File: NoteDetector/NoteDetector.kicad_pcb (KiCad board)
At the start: 2 copper layers, 25 x 25 mm, 24 parts, among them J1 Conn_02x03, J3 Conn_01x01, J4 Conn_01x01, Q1 Q_NMOS_DGS, U1 VM1010, U2 OPAMP, U3 ATtiny1614-SS

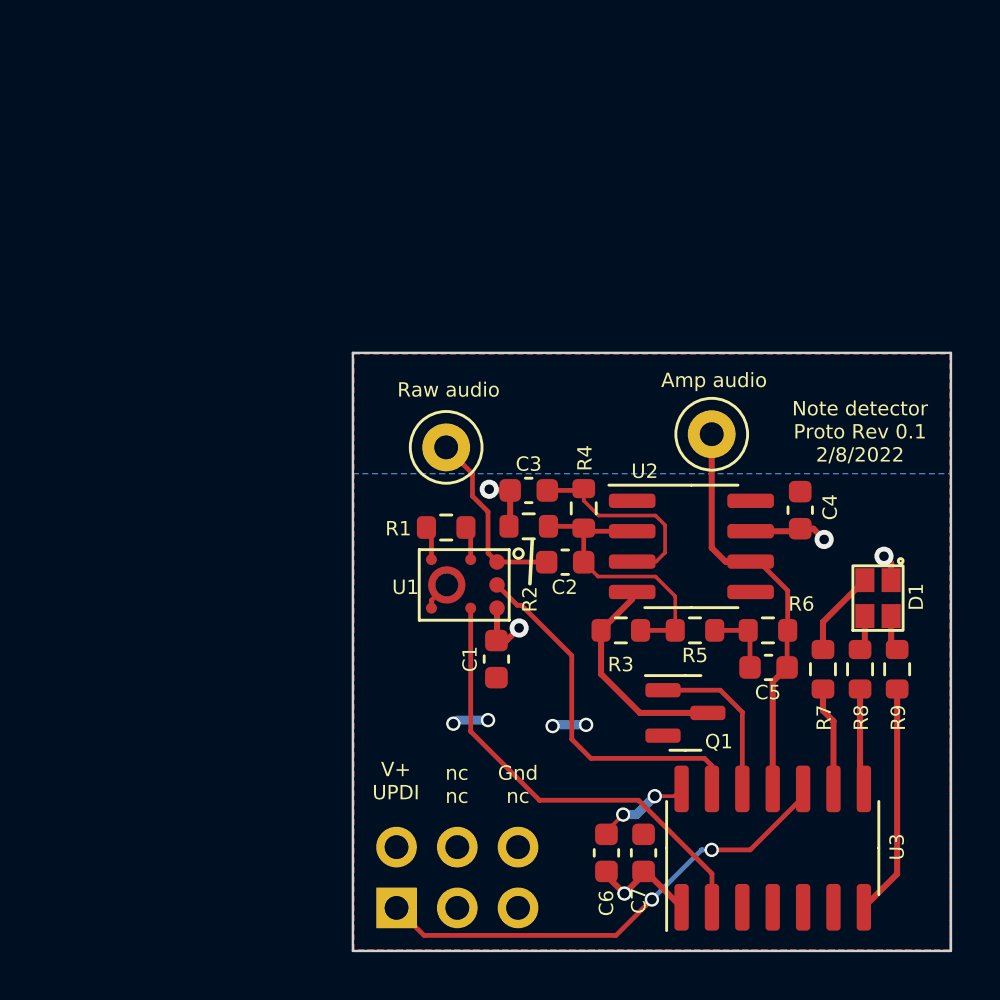
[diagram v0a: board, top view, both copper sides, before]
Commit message: save work: new layout almost done
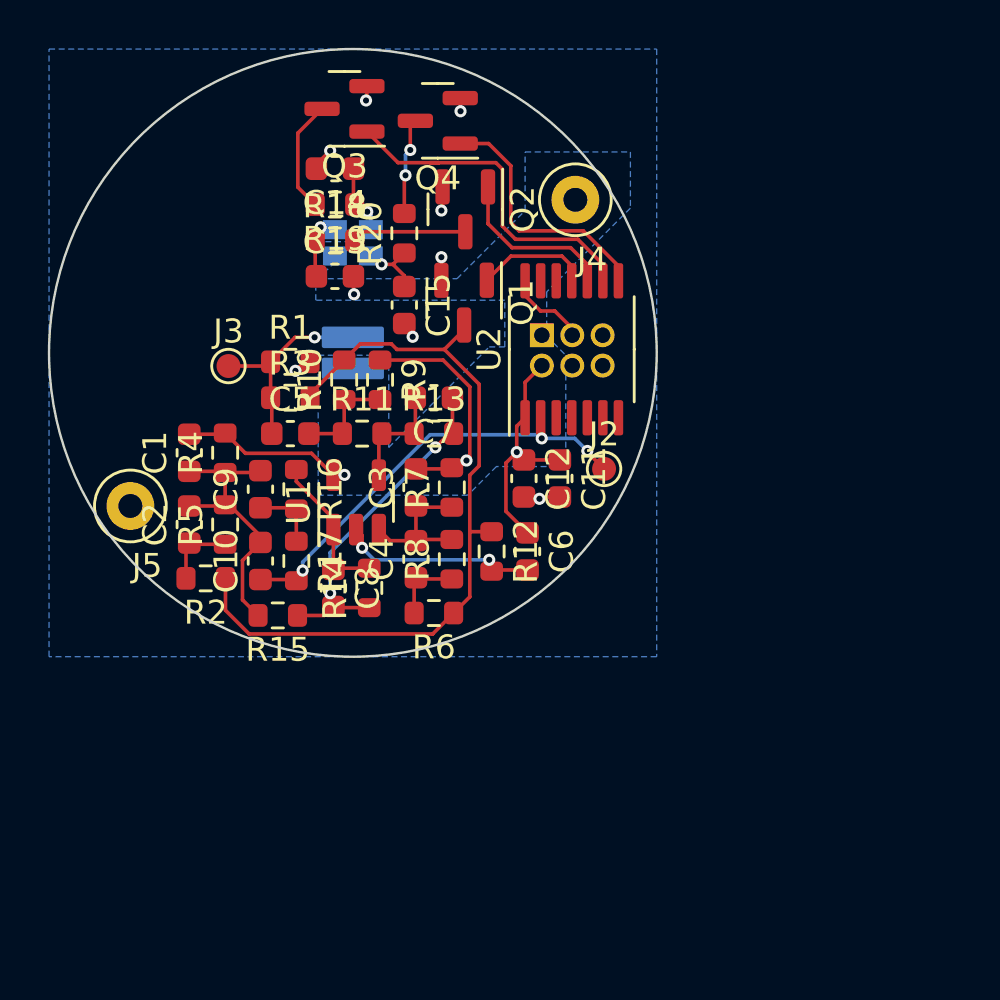
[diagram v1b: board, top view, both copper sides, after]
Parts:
- removed U3: ATtiny1614-SS, Package_SO:SOIC-14_3.9x8.7mm_P1.27mm
- added C10: 22p, Capacitor_SMD:C_0603_1608Metric, F.Cu at (-3.86, 8.70)
- added C11: 100n, Capacitor_SMD:C_0603_1608Metric, F.Cu at (8.65, 5.25)
- added C12: 10n, Capacitor_SMD:C_0603_1608Metric, F.Cu at (7.15, 5.25)
- added C13: 1u, Capacitor_SMD:C_0603_1608Metric, F.Cu at (-0.75, -3.20)
- added C14: 1u, Capacitor_SMD:C_0603_1608Metric, F.Cu at (-0.75, -7.70)
- added C15: 1u, Capacitor_SMD:C_0603_1608Metric, F.Cu at (2.15, -2.00)
- added C8: 22p, Capacitor_SMD:C_0603_1608Metric, F.Cu at (-0.81, 9.82)
- added C9: 22p, Capacitor_SMD:C_0603_1608Metric, F.Cu at (-3.86, 5.70)
- added J2: Conn_01x01, TestPoint:TestPoint_Pad_D1.0mm, F.Cu at (10.5, 4.85)
- added J5: Conn_01x01, TestPoint:TestPoint_Loop_D2.50mm_Drill1.0mm, F.Cu at (-9.30, 6.40)
- added MK1: Microphone_Condenser, User:ElectretCondenserMic_SMT_MO063602-1, B.Cu at (0.00, 0.00)
- added Q2: Q_NMOS_DGS, Package_TO_SOT_SMD:SOT-23, F.Cu at (4.70, -6.00)
- added Q3: Q_NMOS_DGS, Package_TO_SOT_SMD:SOT-23, F.Cu at (-0.35, -10.2)
- added Q4: Q_NMOS_DGS, Package_TO_SOT_SMD:SOT-23, F.Cu at (3.55, -9.70)
- added R10: 10M, Resistor_SMD:R_0603_1608Metric, F.Cu at (-0.36, 1.12)
- added R11: 270k, Resistor_SMD:R_0603_1608Metric, F.Cu at (0.39, 3.38)
- added R12: 100, Resistor_SMD:R_0603_1608Metric, F.Cu at (5.80, 8.30)
- added R13: 10M, Resistor_SMD:R_0603_1608Metric, F.Cu at (3.39, 3.38)
- added R14: 10M, Resistor_SMD:R_0603_1608Metric, F.Cu at (0.69, 9.82)
- added R15: 270k, Resistor_SMD:R_0603_1608Metric, F.Cu at (-3.14, 11.0)
- added R16: 270k, Resistor_SMD:R_0603_1608Metric, F.Cu at (-2.36, 5.70)
- added R17: 270k, Resistor_SMD:R_0603_1608Metric, F.Cu at (-2.36, 8.70)
- added R18: R, Resistor_SMD:R_0603_1608Metric, F.Cu at (-0.75, -4.70)
- added R19: R, Resistor_SMD:R_0603_1608Metric, F.Cu at (-0.75, -6.20)
- added R20: R, Resistor_SMD:R_0603_1608Metric, F.Cu at (2.15, -5.00)
- C1, C4: value 100n -> 1n
- C2: value 1.5n -> 1n
- C3: value C -> 1n
- C5: value 47p -> 100n
- C6: value 100n -> 10n
- C7: value 10n -> 22p
- D1: moved to B.Cu
- J1: value Conn_02x03 -> Conn_01x05; footprint Connector_PinSocket_2.54mm:PinSocket_2x03_P2.54mm_Vertical -> Connector_PinHeader_1.27mm:PinHeader_2x03_P1.27mm_Vertical
- J3: footprint TestPoint:TestPoint_Loop_D2.50mm_Drill1.0mm -> TestPoint:TestPoint_Pad_D1.0mm
- R1: value 18k -> 1k
- R2, R3: value 10M -> 1k
- R5: value 10k -> 10M
- R6: value 1M -> 1k
- R7, R8, R9: value R -> 10M
- U1: value VM1010 -> OPAMP; footprint User:MEMS_mic_VS1010 -> Package_TO_SOT_SMD:SOT-23-5
- U2: value OPAMP -> PIC18F06; footprint Package_SO:SOIC-8_3.9x4.9mm_P1.27mm -> Package_SO:TSSOP-14_4.4x5mm_P0.65mm
- moved D1 26.5 mm to (0.00, -4.60), turned to 180 degrees
- moved R9 24.8 mm to (1.14, 1.12)
- moved J1 24.7 mm to (7.90, -0.74)
- moved C5 22.3 mm to (-2.61, 3.38), turned to 0 degrees
- moved C7 20.9 mm to (3.39, 1.88), turned to 180 degrees
- moved J3 20.4 mm to (-5.20, 0.55)
- moved R5 20.1 mm to (-5.34, 7.17), turned to 90 degrees
- moved Q1 19.5 mm to (4.65, -2.10), turned to -90 degrees
- moved R8 17.7 mm to (4.14, 8.62), turned to 90 degrees
- moved R7 17.3 mm to (4.14, 5.62), turned to 90 degrees
- moved R3 16.9 mm to (-2.61, 1.88), turned to 0 degrees
- moved C4 16.2 mm to (2.64, 8.62), turned to 90 degrees
- moved C2 15.8 mm to (-6.84, 7.17), turned to 90 degrees
- moved C1 15.5 mm to (-6.84, 4.17)
- moved R4 15.2 mm to (-5.34, 4.17)
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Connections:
- C1 pad 1: GND -> /Midscale2
- C2 pad 1: /Audio_raw -> Net-(C2-Pad1)
- C2 pad 2: Net-(C2-Pad2) -> /Midscale2
- C3 pad 1: Net-(C3-Pad1) -> /Midscale1
- C4 pad 1: GND -> Net-(C4-Pad1)
- C4 pad 2: +BATT -> /Midscale1
- C5 pad 1: /Audio_In -> /Audio_raw
- C6 pad 2: GND -> Net-(C6-Pad2)
- C7 pad 1: +BATT -> Net-(C7-Pad1)
- C7 pad 2: GND -> Net-(C7-Pad2)
- J1 pad 1: /UPDI -> /~{MCLR}
- J1 pad 3: unconnected-(J1-Pad3) -> GND
- J1 pad 4: unconnected-(J1-Pad4) -> /ICSP_DAT
- J1 pad 5: unconnected-(J1-Pad5) -> /ICSP_CLK
- J1 pad 6: GND -> unconnected-(J1-Pad6)
- J3 pad 1: /Audio_In -> /Audio_raw
- J4 pad 1: /Audio_raw -> +BATT
- Q1 pad 3: /AFE_gnd -> /gnd_switch
- R1 pad 1: Net-(R1-Pad1) -> /Audio_raw
- R1 pad 2: Net-(R1-Pad2) -> GND
- R2 pad 1: +BATT -> /gnd_switch
- R2 pad 2: Net-(C2-Pad2) -> Net-(C2-Pad1)
- R3 pad 1: Net-(C2-Pad2) -> /Audio_raw
- R3 pad 2: /AFE_gnd -> /gnd_switch
- R4 pad 1: Net-(C2-Pad2) -> /Midscale2
- R4 pad 2: Net-(C3-Pad1) -> +BATT
- R5 pad 1: Net-(C2-Pad2) -> Net-(C2-Pad1)
- R5 pad 2: Net-(C5-Pad2) -> /Midscale2
- R6 pad 1: Net-(C5-Pad2) -> /gnd_switch
- R6 pad 2: /Audio_In -> Net-(C4-Pad1)
- R7 pad 1: Net-(D1-Pad4) -> /Midscale1
- R7 pad 2: /PWM1 -> +BATT
- R8 pad 1: Net-(D1-Pad3) -> Net-(C4-Pad1)
- R8 pad 2: /PWM2 -> /Midscale1
- R9 pad 1: Net-(D1-Pad2) -> +BATT
- R9 pad 2: /PWM3 -> Net-(C5-Pad2)
- U1 pad 1: /Audio_raw -> Net-(C8-Pad1)
- U1 pad 2: Net-(R1-Pad1) -> Net-(C6-Pad2)
- U1 pad 3: Net-(R1-Pad2) -> /Midscale1
- U1 pad 4: GND -> Net-(C7-Pad2)
- U1 pad 5: /Mic_En -> +BATT
- U2 pad 1: unconnected-(U2-Pad1) -> +BATT
- U2 pad 2: Net-(C2-Pad2) -> /Audio_In
- U2 pad 3: Net-(C3-Pad1) -> unconnected-(U2-Pad3)
- U2 pad 4: /AFE_gnd -> /~{MCLR}
- U2 pad 6: /Audio_In -> unconnected-(U2-Pad6)
- U2 pad 7: +BATT -> unconnected-(U2-Pad7)
- U2 pad 8: unconnected-(U2-Pad8) -> /PWM3
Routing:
- net /gnd_switch: track 0.00 -> 32.7 mm
- net /UPDI: track 20.2 -> 0.00 mm, vias 2 -> 0
- net /Mic_En: track 19.2 -> 0.00 mm
- net /Wake: track 15.5 -> 0.00 mm
- net Net-(C7-Pad1): track 0.00 -> 14.2 mm, vias 0 -> 2
- net +BATT: track 14.1 -> 26.8 mm, vias 5 -> 3
- net Net-(C2-Pad2): track 12.3 -> 0.00 mm
- net /Midscale2: track 0.00 -> 11.8 mm
- net /PWM2: track 4.24 -> 14.6 mm
- net /AFE_gnd: track 9.10 -> 0.00 mm
- net Net-(C3-Pad1): track 8.56 -> 0.00 mm
- net Net-(C6-Pad2): track 0.00 -> 8.42 mm, vias 0 -> 2
- net Net-(C8-Pad1): track 0.00 -> 6.34 mm
- net /Midscale1: track 0.00 -> 6.23 mm
- net Net-(R18-Pad2): track 0.00 -> 4.78 mm
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- added copper zone on B.Cu, net GND
- removed copper zone on F.Cu, net GND
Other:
- board size 25 x 25 mm -> 25.4 x 25.4 mm
- board text removed: "Amp audio"
- board text removed: "Gnd nc"
- board text removed: "Note detector Proto Rev 0.1 2/8/2022"
- board text removed: "Raw audio"
- board text removed: "V+ UPDI"
- board text removed: "nc nc"
